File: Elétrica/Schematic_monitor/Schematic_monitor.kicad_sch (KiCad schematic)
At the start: 63 parts, among them J1 Conn_01x04, J2 USB_B_Micro, J3 Eletrode 1, J4 Eletrode 2, J5 Conn_01x09, SW1 SW_Push, SW2 SW_SPDT, U1 STM32F446RET6TR, U2 LM1117S-3.3, U3 MLX90614ESF-ACC-000-TU, U4 MAX30100EFD+, U5 AD623, U6 LM358, U7 LM358, U8 LM358, Y1 Crystal_25MHz

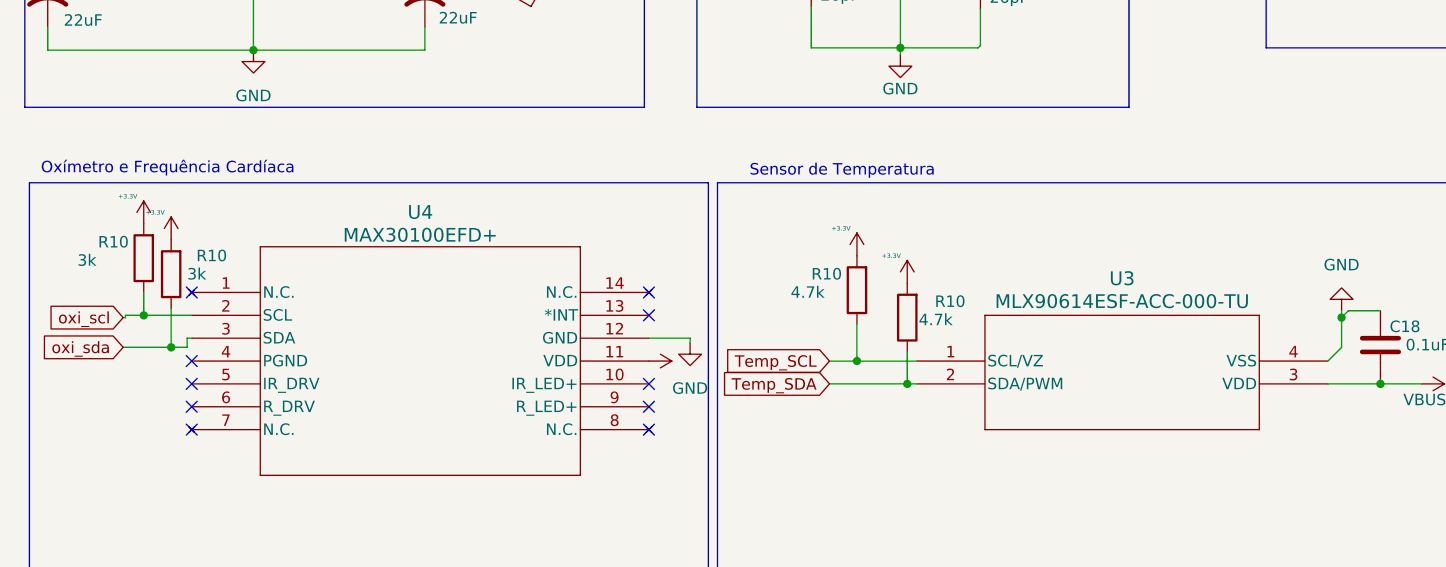
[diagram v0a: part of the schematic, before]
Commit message: PRJ4
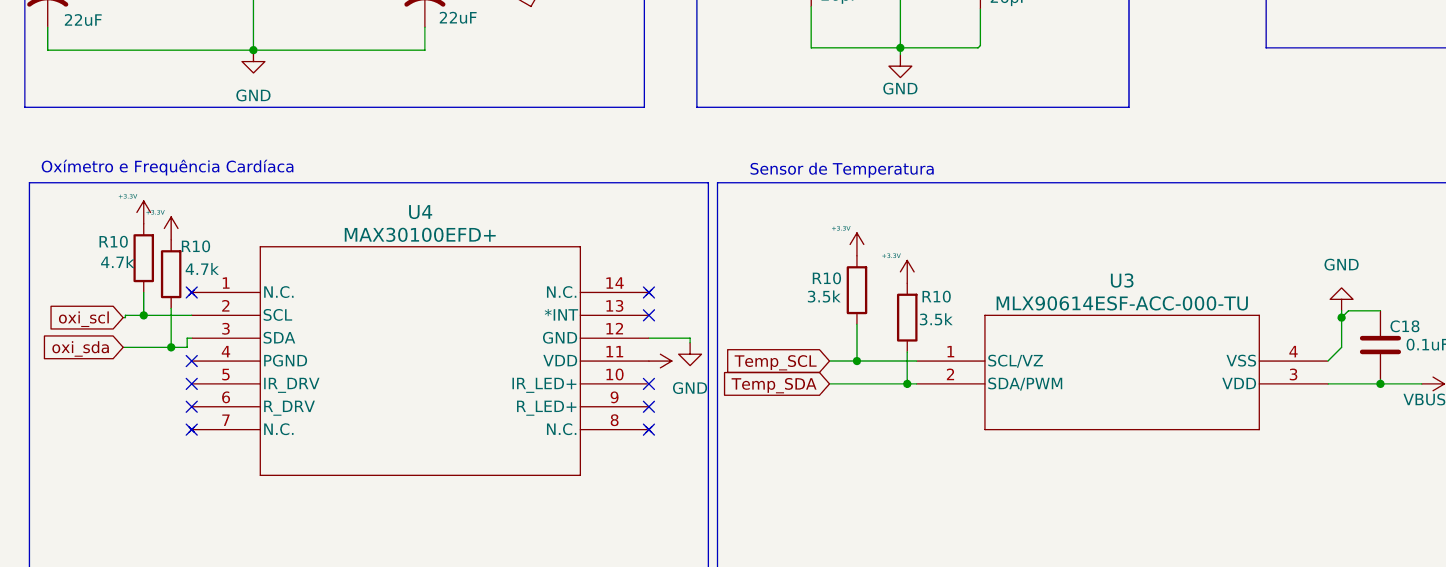
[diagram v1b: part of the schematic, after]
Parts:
- R10: value 3k -> 4.7k
- R10: value 4.7k -> 3.5k
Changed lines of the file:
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@@
       (effects (font (size 1.27 1.27)) (justify right))
     )
-    (property "Value" "3k" (at 19.558 146.304 0)
+    (property "Value" "4.7k" (at 22.098 146.558 0)
       (effects (font (size 1.27 1.27)) (justify right))
     )
@@
   (symbol (lib_id "Device:R") (at 111.76 152.654 180) (unit 1)
     (in_bom yes) (on_board yes) (dnp no)
-    (property "Reference" "R10" (at 114.808 150.876 0)
+    (property "Reference" "R10" (at 113.284 150.368 0)
       (effects (font (size 1.27 1.27)) (justify right))
     )
-    (property "Value" "4.7k" (at 113.03 152.908 0)
+    (property "Value" "3.5k" (at 113.03 152.908 0)
       (effects (font (size 1.27 1.27)) (justify right))
     )
@@
   (symbol (lib_id "Temp_sensor:MLX90614ESF-ACC-000-TU") (at 112.776 157.48 0) (unit 1)
     (in_bom yes) (on_board yes) (dnp no) (fields_autoplaced)
-    (property "Reference" "U3" (at 135.636 148.336 0)
+    (property "Reference" "U3" (at 135.636 148.59 0)
       (effects (font (size 1.524 1.524)))
     )
-    (property "Value" "MLX90614ESF-ACC-000-TU" (at 135.636 150.876 0)
+    (property "Value" "MLX90614ESF-ACC-000-TU" (at 135.636 151.13 0)
       (effects (font (size 1.524 1.524)))
     )
@@
   (symbol (lib_id "Device:R") (at 106.172 149.606 180) (unit 1)
     (in_bom yes) (on_board yes) (dnp no)
-    (property "Reference" "R10" (at 101.092 147.828 0)
+    (property "Reference" "R10" (at 101.092 148.336 0)
       (effects (font (size 1.27 1.27)) (justify right))
     )
-    (property "Value" "4.7k" (at 98.806 149.86 0)
+    (property "Value" "3.5k" (at 100.584 150.368 0)
       (effects (font (size 1.27 1.27)) (justify right))
     )
@@
   (symbol (lib_id "Device:R") (at 29.972 147.828 180) (unit 1)
     (in_bom yes) (on_board yes) (dnp no)
-    (property "Reference" "R10" (at 32.766 145.796 0)
+    (property "Reference" "R10" (at 30.988 144.78 0)
       (effects (font (size 1.27 1.27)) (justify right))
     )
-    (property "Value" "3k" (at 31.75 147.828 0)
+    (property "Value" "4.7k" (at 31.496 147.32 0)
       (effects (font (size 1.27 1.27)) (justify right))
     )

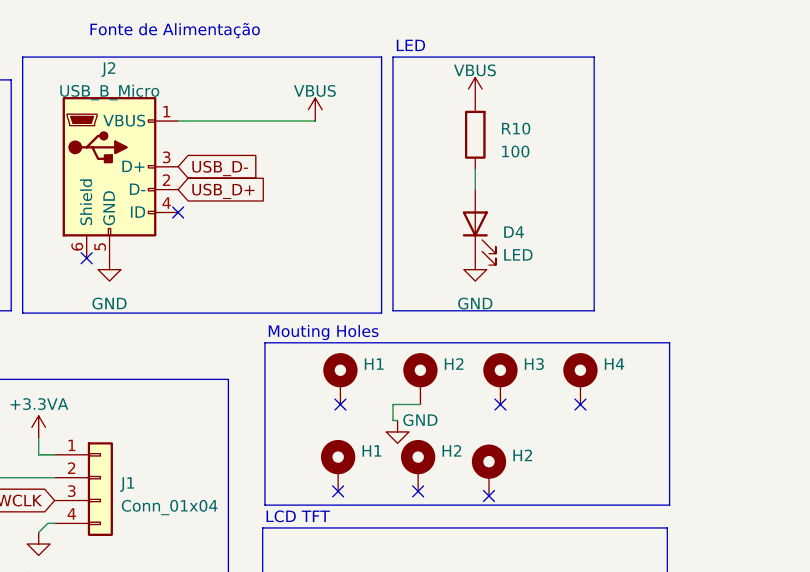
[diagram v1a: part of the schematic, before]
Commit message: PRJ4
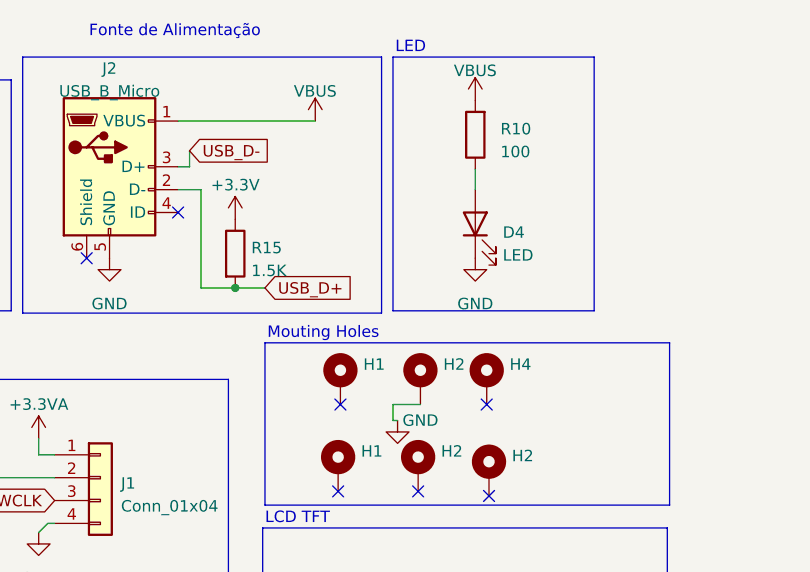
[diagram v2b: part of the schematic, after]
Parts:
- removed H3: MountingHole_Pad, MountingHole:MountingHole_2.2mm_M2_DIN965_Pad, symbol Mechanical:MountingHole_Pad
- added R15: 1.5K, Resistor_SMD:R_0603_1608Metric_Pad0.98x0.95mm_HandSolder, symbol Device:R
- C5: footprint Capacitor_SMD:C_0603_1608Metric -> Capacitor_SMD:C_0805_2012Metric_Pad1.18x1.45mm_HandSolder
- C6, C7: footprint Capacitor_SMD:C_0603_1608Metric -> Capacitor_SMD:CP_Elec_3x5.3
- FB1: footprint Inductor_SMD:L_0603_1608Metric_Pad1.05x0.95mm_HandSolder -> Inductor_SMD:L_0805_2012Metric
- H1, H2, H4: footprint MountingHole:MountingHole_2.2mm_M2_DIN965_Pad -> MountingHole:MountingHole_3.2mm_M3
- U3: footprint temp:MLX90614xCC_MEL -> Oscillator:Oscillator_SMD_TXC_7C-4Pin_5.0x3.2mm
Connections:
- net +3.3V: now also R15.1
- net USB_D+: now also R15.2
- no-connect marks 49 -> 48
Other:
- moved on the sheet: H4
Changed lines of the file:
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@@
   (junction (at 107.95 203.2) (diameter 0) (color 0 0 0 0)
   )
+  (junction (at 148.59 51.054) (diameter 0) (color 0 0 0 0)
+  )
   (junction (at 25.4 33.02) (diameter 0) (color 0 0 0 0)
   )
@@
   (no_connect (at 238.506 206.502))
   (no_connect (at 202.946 181.102))
-  (no_connect (at 178.054 64.008))
   (no_connect (at 32.258 160.02))
   (no_connect (at 202.946 170.942))
-  (no_connect (at 142.24 42.672))
   (no_connect (at 176.784 74.168))
-  (no_connect (at 186.944 64.008))
+  (no_connect (at 176.53 64.008))
   (no_connect (at 202.946 191.262))
   (no_connect (at 238.506 201.422))
@@
   (no_connect (at 83.058 152.4))
   (no_connect (at 202.946 186.182))
+  (no_connect (at 142.24 42.672))
   (no_connect (at 238.506 196.342))
   (no_connect (at 202.946 165.862))
@@
     (stroke (width 0) (type default))
   )
+  (wire (pts (xy 142.24 40.132) (xy 144.78 40.132))
+    (stroke (width 0) (type default))
+  )
   (wire (pts (xy 119.126 96.266) (xy 119.126 97.79))
     (stroke (width 0) (type default))
@@
     (stroke (width 0) (type default))
   )
+  (wire (pts (xy 143.51 35.814) (xy 143.51 37.592))
+    (stroke (width 0) (type default))
+  )
   (wire (pts (xy 60.706 74.168) (xy 61.976 72.898))
     (stroke (width 0) (type default))
@@
     (stroke (width 0) (type default))
   )
+  (wire (pts (xy 144.78 51.054) (xy 148.59 51.054))
+    (stroke (width 0) (type default))
+  )
+  (wire (pts (xy 148.59 51.054) (xy 151.892 51.054))
+    (stroke (width 0) (type default))
+  )
   (wire (pts (xy 110.998 122.682) (xy 119.634 122.682))
     (stroke (width 0) (type default))
@@
     (stroke (width 0) (type default))
   )
+  (wire (pts (xy 143.51 37.592) (xy 142.24 37.592))
+    (stroke (width 0) (type default))
+  )
   (wire (pts (xy 25.4 44.45) (xy 35.56 44.45))
     (stroke (width 0) (type default))
@@
     (stroke (width 0) (type default))
   )
+  (wire (pts (xy 144.78 40.132) (xy 144.78 51.054))
+    (stroke (width 0) (type default))
+  )
   (wire (pts (xy 65.278 200.914) (xy 68.834 200.914))
     (stroke (width 0) (type default))
@@
     )
   )
-  (global_label "USB_D-" (shape input) (at 142.24 37.592 0) (fields_autoplaced)
+  (global_label "USB_D-" (shape input) (at 143.51 35.814 0) (fields_autoplaced)
     (effects (font (size 1.27 1.27)) (justify left))
-    (property "Intersheetrefs" "${INTERSHEET_REFS}" (at 152.7658 37.592 0)
+    (property "Intersheetrefs" "${INTERSHEET_REFS}" (at 154.0358 35.814 0)
       (effects (font (size 1.27 1.27)) (justify left) hide)
     )
@@
     )
   )
-  (global_label "USB_D+" (shape input) (at 142.24 40.132 0) (fields_autoplaced)
+  (global_label "USB_D+" (shape input) (at 151.892 51.054 0) (fields_autoplaced)
     (effects (font (size 1.27 1.27)) (justify left))
-    (property "Intersheetrefs" "${INTERSHEET_REFS}" (at 152.7658 40.132 0)
+    (property "Intersheetrefs" "${INTERSHEET_REFS}" (at 162.4178 51.054 0)
       (effects (font (size 1.27 1.27)) (justify left) hide)
     )
@@
       (effects (font (size 1.27 1.27)) (justify left) hide)
     )
-    (property "Footprint" "MountingHole:MountingHole_2.2mm_M2_DIN965_Pad" (at 169.164 61.468 0)
+    (property "Footprint" "MountingHole:MountingHole_3.2mm_M3" (at 169.164 61.468 0)
       (effects (font (size 1.27 1.27)) hide)
     )
@@
       (effects (font (size 1.27 1.27)) (justify left))
     )
-    (property "Footprint" "Capacitor_SMD:C_0603_1608Metric" (at 16.256 116.586 0)
+    (property "Footprint" "Capacitor_SMD:CP_Elec_3x5.3" (at 16.256 116.586 0)
       (effects (font (size 1.27 1.27)) hide)
     )
@@
       (effects (font (size 1.27 1.27)) (justify left) hide)
     )
-    (property "Footprint" "MountingHole:MountingHole_2.2mm_M2_DIN965_Pad" (at 176.784 71.628 0)
+    (property "Footprint" "MountingHole:MountingHole_3.2mm_M3" (at 176.784 71.628 0)
       (effects (font (size 1.27 1.27)) hide)
     )
@@
     )
   )
-  (symbol (lib_id "Mechanical:MountingHole_Pad") (at 178.054 61.468 0) (unit 1)
-    (in_bom yes) (on_board yes) (dnp no) (fields_autoplaced)
-    (property "Reference" "H3" (at 180.594 59.563 0)
-      (effects (font (size 1.27 1.27)) (justify left))
-    )
-    (property "Value" "MountingHole_Pad" (at 180.594 62.103 0)
-      (effects (font (size 1.27 1.27)) (justify left) hide)
-    )
-    (property "Footprint" "MountingHole:MountingHole_2.2mm_M2_DIN965_Pad" (at 178.054 61.468 0)
-      (effects (font (size 1.27 1.27)) hide)
-    )
-    (property "Datasheet" "~" (at 178.054 61.468 0)
-      (effects (font (size 1.27 1.27)) hide)
-    )
-    (pin "1")
-    (instances
-      (project "ProjetoSEMB_Gabriel_Rafael"
-        (path "/71af4175-d518-4051-8306-cd60f2e5793a"
-          (reference "H3") (unit 1)
-        )
-      )
-      (project "Schematic_monitor"
-        (path "/e9cd3b8d-6ac1-4cca-9ad1-0be06fd7b6c7"
-          (reference "H5") (unit 1)
-        )
-      )
-    )
-  )
   (symbol (lib_id "power:+3.3V") (at 45.466 66.548 0) (unit 1)
     (in_bom yes) (on_board yes) (dnp no) (fields_autoplaced)
@@
       (effects (font (size 1.27 1.27)) hide)
     )
-    (property "Footprint" "Inductor_SMD:L_0603_1608Metric_Pad1.05x0.95mm_HandSolder" (at 38.354 66.802 90)
+    (property "Footprint" "Inductor_SMD:L_0805_2012Metric" (at 38.354 66.802 90)
       (effects (font (size 1.27 1.27)) hide)
     )
@@
       (effects (font (size 1.27 1.27)) (justify left))
     )
-    (property "Footprint" "MountingHole:MountingHole_2.2mm_M2_DIN965_Pad" (at 160.274 61.468 0)
+    (property "Footprint" "MountingHole:MountingHole_3.2mm_M3" (at 160.274 61.468 0)
       (effects (font (size 1.27 1.27)) hide)
     )
@@
     )
   )
-  (symbol (lib_id "Mechanical:MountingHole_Pad") (at 186.944 61.468 0) (unit 1)
+  (symbol (lib_id "Mechanical:MountingHole_Pad") (at 176.53 61.468 0) (unit 1)
     (in_bom yes) (on_board yes) (dnp no) (fields_autoplaced)
-    (property "Reference" "H4" (at 189.484 59.563 0)
+    (property "Reference" "H4" (at 179.07 59.563 0)
       (effects (font (size 1.27 1.27)) (justify left))
     )
-    (property "Value" "MountingHole_Pad" (at 189.484 62.103 0)
+    (property "Value" "MountingHole_Pad" (at 179.07 62.103 0)
       (effects (font (size 1.27 1.27)) (justify left) hide)
     )
-    (property "Footprint" "MountingHole:MountingHole_2.2mm_M2_DIN965_Pad" (at 186.944 61.468 0)
+    (property "Footprint" "MountingHole:MountingHole_3.2mm_M3" (at 176.53 61.468 0)
       (effects (font (size 1.27 1.27)) hide)
     )
-    (property "Datasheet" "~" (at 186.944 61.468 0)
+    (property "Datasheet" "~" (at 176.53 61.468 0)
       (effects (font (size 1.27 1.27)) hide)
     )
@@
       (effects (font (size 1.27 1.27)) (justify left) hide)
     )
-    (property "Footprint" "MountingHole:MountingHole_2.2mm_M2_DIN965_Pad" (at 168.91 71.12 0)
+    (property "Footprint" "MountingHole:MountingHole_3.2mm_M3" (at 168.91 71.12 0)
       (effects (font (size 1.27 1.27)) hide)
     )
@@
       (effects (font (size 1.27 1.27)) (justify left))
     )
-    (property "Footprint" "Capacitor_SMD:C_0603_1608Metric" (at 16.4592 40.64 0)
+    (property "Footprint" "Capacitor_SMD:C_0805_2012Metric_Pad1.18x1.45mm_HandSolder" (at 16.4592 40.64 0)
       (effects (font (size 1.27 1.27)) hide)
     )
@@
       (effects (font (size 1.27 1.27)) (justify left) hide)
     )
-    (property "Footprint" "MountingHole:MountingHole_2.2mm_M2_DIN965_Pad" (at 160.02 71.12 0)
+    (property "Footprint" "MountingHole:MountingHole_3.2mm_M3" (at 160.02 71.12 0)
       (effects (font (size 1.27 1.27)) hide)
     )
@@
       (effects (font (size 1.524 1.524)))
     )
-    (property "Footprint" "temp:MLX90614xCC_MEL" (at 112.776 157.48 0)
+    (property "Footprint" "Oscillator:Oscillator_SMD_TXC_7C-4Pin_5.0x3.2mm" (at 112.776 157.48 0)
       (effects (font (size 1.27 1.27) italic) hide)
     )
@@
     )
   )
+  (symbol (lib_id "Device:R") (at 148.59 47.244 0) (unit 1)
+    (in_bom yes) (on_board yes) (dnp no) (fields_autoplaced)
+    (property "Reference" "R15" (at 150.368 46.609 0)
+      (effects (font (size 1.27 1.27)) (justify left))
+    )
+    (property "Value" "1.5K" (at 150.368 49.149 0)
+      (effects (font (size 1.27 1.27)) (justify left))
+    )
+    (property "Footprint" "Resistor_SMD:R_0603_1608Metric_Pad0.98x0.95mm_HandSolder" (at 146.812 47.244 90)
+      (effects (font (size 1.27 1.27)) hide)
+    )
+    (property "Datasheet" "~" (at 148.59 47.244 0)
+      (effects (font (size 1.27 1.27)) hide)
+    )
+    (pin "1")
+    (pin "2")
+    (instances
+      (project "Schematic_monitor"
+        (path "/e9cd3b8d-6ac1-4cca-9ad1-0be06fd7b6c7"
+          (reference "R15") (unit 1)
+        )
+      )
+    )
+  )
   (symbol (lib_id "power:+3.3V") (at 26.924 142.24 0) (unit 1)
     (in_bom yes) (on_board yes) (dnp no)
@@
       (effects (font (size 1.27 1.27)) (justify left))
     )
-    (property "Footprint" "Capacitor_SMD:C_0603_1608Metric" (at 58.166 116.586 0)
+    (property "Footprint" "Capacitor_SMD:CP_Elec_3x5.3" (at 58.166 116.586 0)
       (effects (font (size 1.27 1.27)) hide)
     )
@@
         )
       )
+    )
+  )
+  (symbol (lib_id "power:+3.3V") (at 148.59 43.434 0) (unit 1)
+    (in_bom yes) (on_board yes) (dnp no) (fields_autoplaced)
+    (property "Reference" "#PWR021" (at 148.59 47.244 0)
+      (effects (font (size 1.27 1.27)) hide)
+    )
+    (property "Value" "+3.3V" (at 148.59 39.624 0)
+      (effects (font (size 1.27 1.27)))
+    )
+    (property "Footprint" "" (at 148.59 43.434 0)
+      (effects (font (size 1.27 1.27)) hide)
+    )
+    (property "Datasheet" "" (at 148.59 43.434 0)
+      (effects (font (size 1.27 1.27)) hide)
+    )
+    (pin "1")
+    (instances
+      (project "ProjetoSEMB_Gabriel_Rafael"
+        (path "/71af4175-d518-4051-8306-cd60f2e5793a"
+          (reference "#PWR021") (unit 1)
+        )
+      )
+      (project "Schematic_monitor"
+        (path "/e9cd3b8d-6ac1-4cca-9ad1-0be06fd7b6c7"
+          (reference "#PWR046") (unit 1)
+        )
+      )
